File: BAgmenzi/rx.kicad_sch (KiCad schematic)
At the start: 30 parts, among them IC1 TPL0501-100RSER, U2 AD8338ACPZ-R7, U3 OPA836IDBVT, U4 OPA836IDBVT

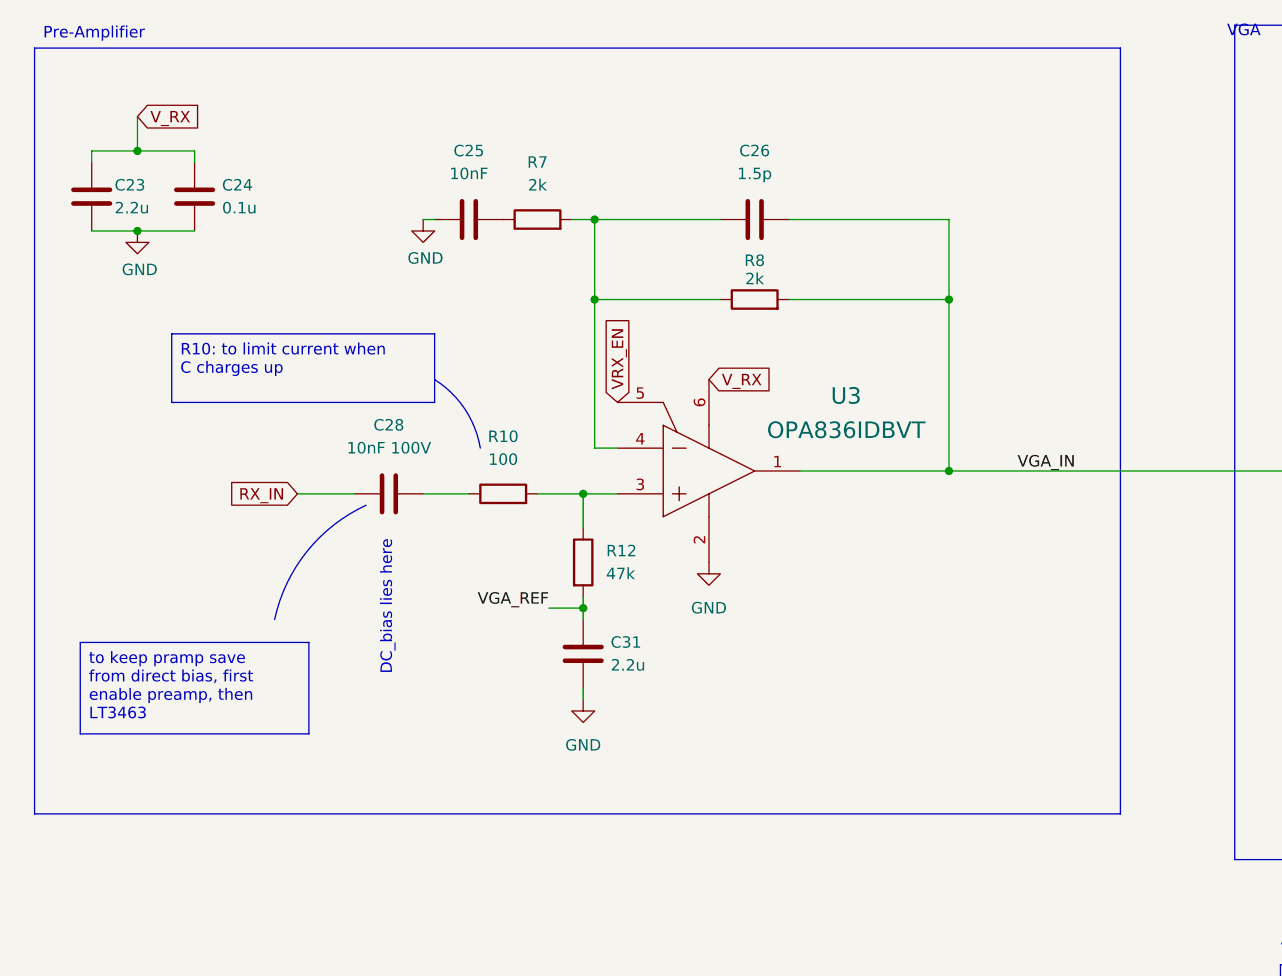
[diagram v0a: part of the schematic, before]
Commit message: started layout, front v backside
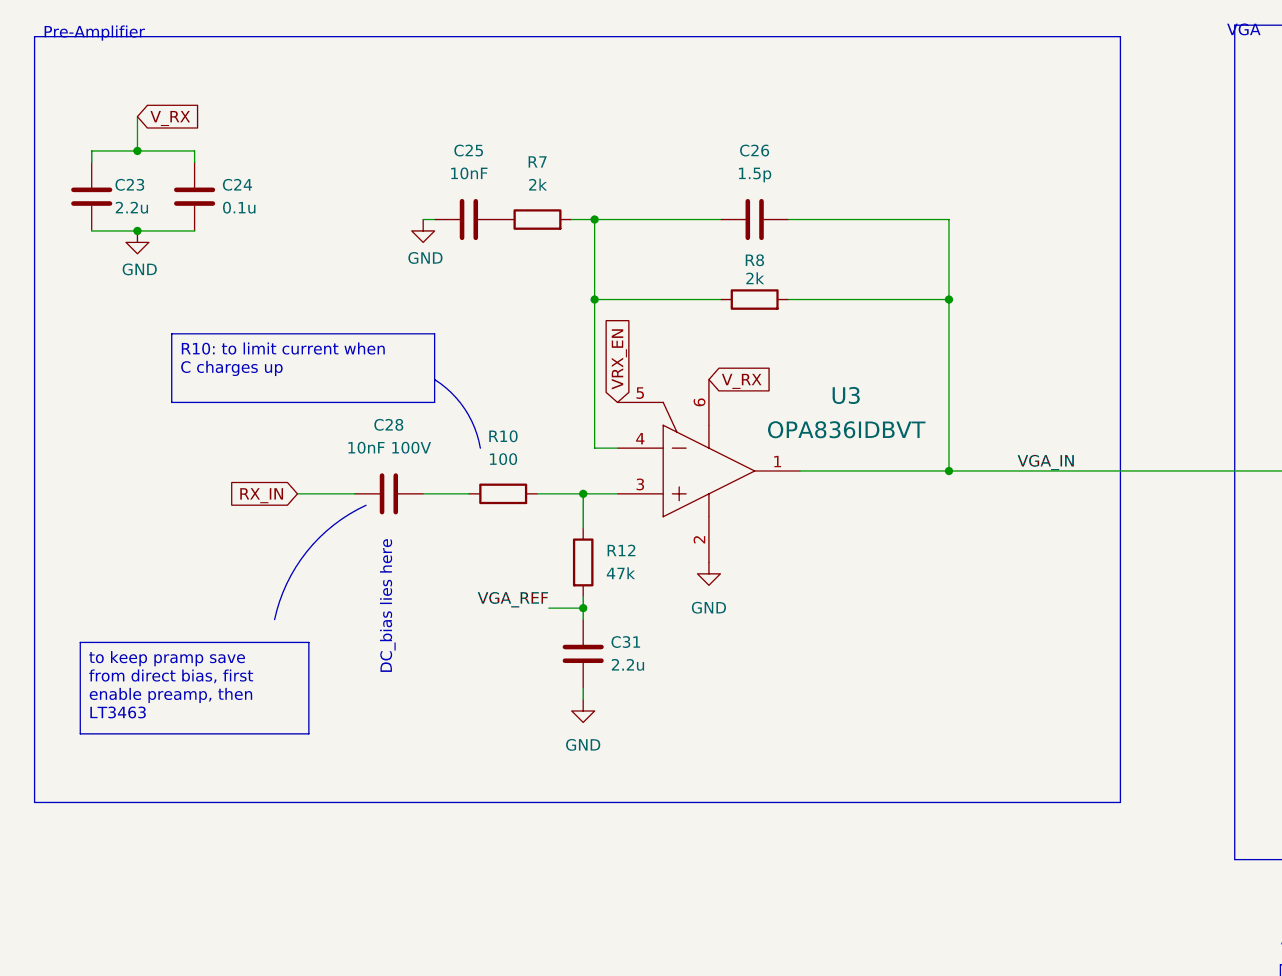
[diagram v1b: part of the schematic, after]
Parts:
- TP2: footprint TestPoint:TestPoint_Loop_D2.50mm_Drill1.85mm -> TestPoint:TestPoint_Pad_D2.0mm
- TP6: footprint TestPoint:TestPoint_Loop_D2.50mm_Drill1.0mm_LowProfile -> TestPoint:TestPoint_Pad_D2.0mm
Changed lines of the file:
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@@
 	)
 	(rectangle
-		(start 19.05 22.86)
-		(end 139.7 107.95)
+		(start 19.05 21.59)
+		(end 139.7 106.68)
 		(stroke
 			(width 0)
@@
 	)
 	(junction
+		(at 120.65 69.85)
+		(diameter 0)
+		(color 0 0 0 0)
+	)
+	(junction
 		(at 80.01 85.09)
 		(diameter 0)
@@
 	)
 	(junction
-		(at 120.65 69.85)
-		(diameter 0)
-		(color 0 0 0 0)
-	)
-	(junction
 		(at 191.77 54.61)
 		(diameter 0)
@@
 			)
 		)
-		(property "Footprint" "TestPoint:TestPoint_Loop_D2.50mm_Drill1.85mm"
+		(property "Footprint" "TestPoint:TestPoint_Pad_D2.0mm"
 			(at 173.99 80.01 0)
 			(effects
@@
 			)
 		)
-		(property "Footprint" "TestPoint:TestPoint_Loop_D2.50mm_Drill1.0mm_LowProfile"
+		(property "Footprint" "TestPoint:TestPoint_Pad_D2.0mm"
 			(at 227.33 151.13 0)
 			(effects
